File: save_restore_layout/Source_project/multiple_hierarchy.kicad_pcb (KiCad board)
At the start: 2 copper layers, 72 parts, among them J1001 Pusa_4mm, J1002 Pusa_4mm, J201 Pusa_4mm, J202 Pusa_4mm, J601 Pusa_4mm, J602 Pusa_4mm, Q1101 CSD19531KCS, Q1102 CSD19531KCS, Q1301 CSD19531KCS, Q1302 CSD19531KCS, Q1401 CSD19531KCS, Q1402 CSD19531KCS, Q301 CSD19531KCS, Q302 CSD19531KCS, Q501 CSD19531KCS, Q502 CSD19531KCS, Q701 CSD19531KCS, Q702 CSD19531KCS, Q901 CSD19531KCS, Q902 CSD19531KCS, U101 TMS320F28027DA, U1101 IR2181, U1201 INA240, U1301 IR2181, U1401 IR2181, U301 IR2181, U401 INA240, U501 IR2181, U701 IR2181, U801 INA240, U901 IR2181

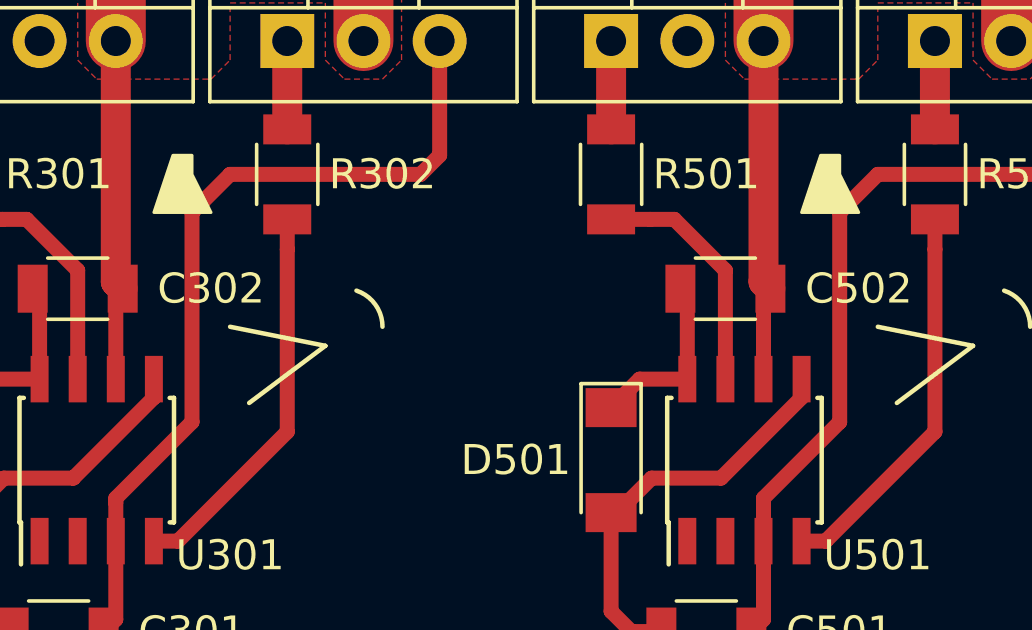
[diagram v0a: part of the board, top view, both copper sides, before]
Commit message: Changed test projects
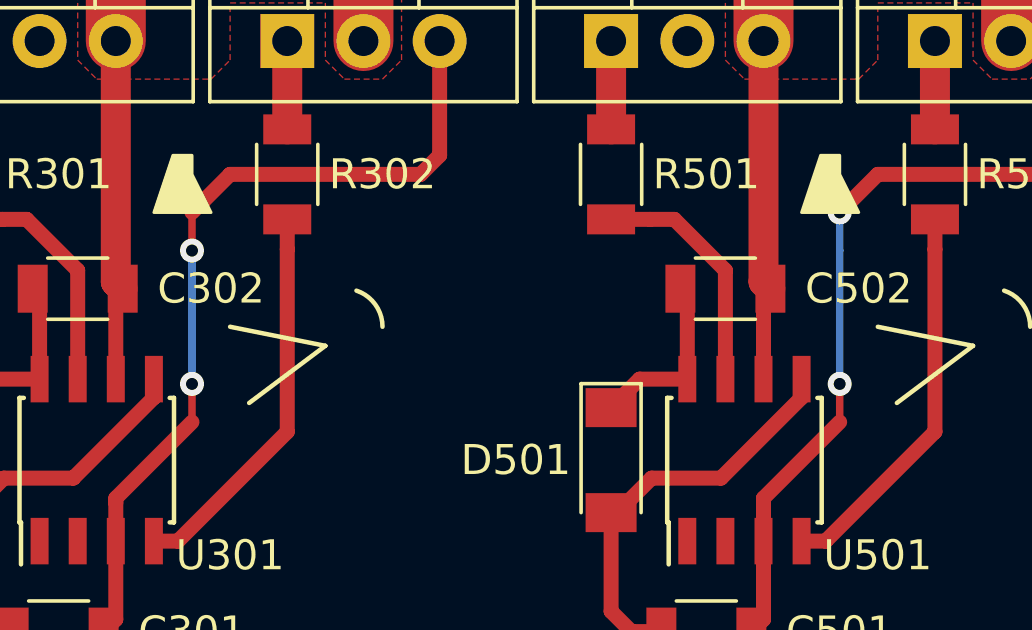
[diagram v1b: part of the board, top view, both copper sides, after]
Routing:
- net -VDC: vias 0 -> 4
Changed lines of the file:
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@@
-(kicad_pcb (version 20171130) (host pcbnew "(5.1.0)-1")
+(kicad_pcb (version 20171130) (host pcbnew "(5.1.2)-1")
   (general
     (thickness 1.6)
     (drawings 18)
-    (tracks 131)
+    (tracks 139)
     (zones 0)
     (modules 72)
@@
   (segment (start 112.395 72.62) (end 111.99 73.025) (width 0.5) (layer F.Cu) (net 14))
   (segment (start 114.935 66.04) (end 112.395 68.58) (width 0.5) (layer F.Cu) (net 14))
-  (segment (start 114.935 59.055) (end 114.935 66.04) (width 0.5) (layer F.Cu) (net 14))
   (segment (start 112.395 68.58) (end 112.395 68.735) (width 0.5) (layer F.Cu) (net 14))
   (segment (start 112.395 68.735) (end 112.395 70.01) (width 0.5) (layer F.Cu) (net 14))
@@
   (segment (start 90.805 68.735) (end 90.805 70.01) (width 0.5) (layer F.Cu) (net 14))
   (segment (start 90.805 68.58) (end 90.805 68.735) (width 0.5) (layer F.Cu) (net 14))
-  (segment (start 93.345 59.055) (end 93.345 66.04) (width 0.5) (layer F.Cu) (net 14))
   (segment (start 93.345 66.04) (end 90.805 68.58) (width 0.5) (layer F.Cu) (net 14))
   (segment (start 90.805 72.62) (end 90.4 73.025) (width 0.5) (layer F.Cu) (net 14))
@@
   (segment (start 186.055 54.135) (end 186.055 53.66) (width 0.5) (layer F.Cu) (net 14))
   (segment (start 186.055 53.66) (end 185.255 52.86) (width 0.5) (layer F.Cu) (net 14))
+  (via (at 93.345 64.77) (size 0.8) (drill 0.4) (layers F.Cu B.Cu) (net 14))
+  (segment (start 93.345 66.04) (end 93.345 64.77) (width 0.25) (layer F.Cu) (net 14))
+  (via (at 93.345 60.325) (size 0.8) (drill 0.4) (layers F.Cu B.Cu) (net 14))
+  (segment (start 93.345 64.77) (end 93.345 60.325) (width 0.25) (layer B.Cu) (net 14))
+  (segment (start 93.345 60.325) (end 93.345 59.055) (width 0.25) (layer F.Cu) (net 14))
+  (via (at 114.935 64.77) (size 0.8) (drill 0.4) (layers F.Cu B.Cu) (net 14))
+  (segment (start 114.935 66.04) (end 114.935 64.77) (width 0.25) (layer F.Cu) (net 14))
+  (segment (start 114.935 64.77) (end 114.935 60.325) (width 0.25) (layer B.Cu) (net 14))
+  (via (at 114.935 59.055) (size 0.8) (drill 0.4) (layers F.Cu B.Cu) (net 14))
+  (segment (start 114.935 60.325) (end 114.935 59.055) (width 0.25) (layer B.Cu) (net 14))
   (segment (start 87.025 59.285) (end 85.725 59.285) (width 0.5) (layer F.Cu) (net 17))
   (segment (start 87.835002 59.285) (end 87.025 59.285) (width 0.5) (layer F.Cu) (net 17))
@@
   (segment (start 114.465 70.01) (end 118.11 66.365) (width 0.5) (layer F.Cu) (net 71))
   (segment (start 113.665 70.01) (end 114.465 70.01) (width 0.5) (layer F.Cu) (net 71))
-  (segment (start 118.11 66.365) (end 118.11 60.285) (width 0.5) (layer F.Cu) (net 71))
   (segment (start 118.11 60.285) (end 118.11 59.285) (width 0.5) (layer F.Cu) (net 71))
+  (segment (start 118.11 66.365) (end 118.11 60.285) (width 0.5) (layer F.Cu) (net 71))
   (segment (start 186.055 46.585) (end 186.285 46.355) (width 0.5) (layer F.Cu) (net 84))
   (segment (start 186.055 48.735) (end 186.055 46.585) (width 0.5) (layer F.Cu) (net 84))
